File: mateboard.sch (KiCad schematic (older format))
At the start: 2 parts, among them J1 IO1, J2 IO2

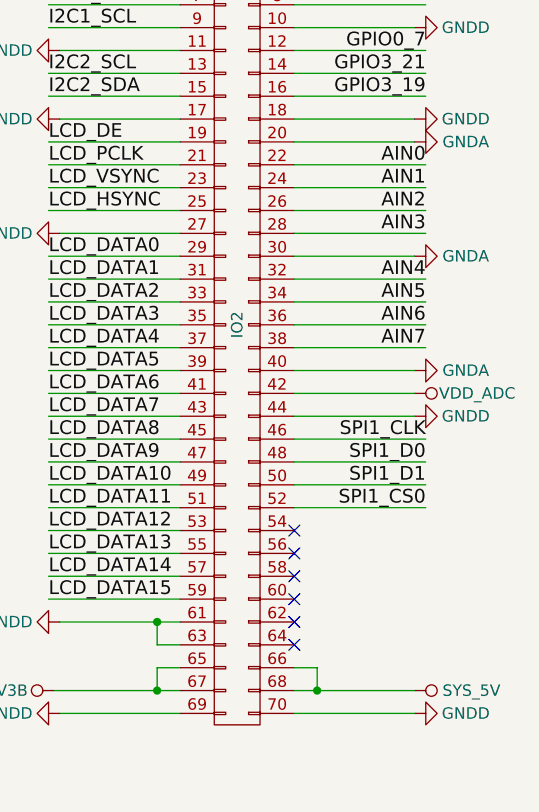
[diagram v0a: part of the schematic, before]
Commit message: erc passed
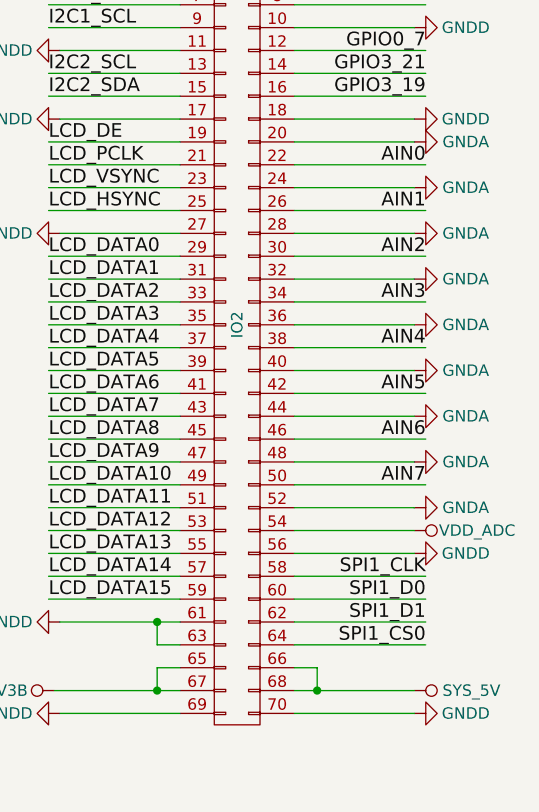
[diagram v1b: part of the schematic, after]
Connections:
- net AIN1: now also J2.26 (P26); no longer J2.24 (P24)
- net AIN2: now also J2.30 (P30); no longer J2.26 (P26)
- net AIN3: now also J2.34 (P34); no longer J2.28 (P28)
- net AIN4: now also J2.38 (P38); no longer J2.32 (P32)
- net AIN5: now also J2.42 (P42); no longer J2.34 (P34)
- net AIN6: now also J2.46 (P46); no longer J2.36 (P36)
- net AIN7: now also J2.50 (P50); no longer J2.38 (P38)
- net GNDA: now also J2.24 (P24), J2.28 (P28), J2.32 (P32), J2.36 (P36), J2.44 (P44), J2.48 (P48), J2.52 (P52); no longer J2.30 (P30)
- net GNDD: now also J2.56 (P56); no longer J2.44 (P44)
- net SPI1_CLK: now also J2.58 (P58); no longer J2.46 (P46)
- net SPI1_CS0: now also J2.64 (P64); no longer J2.52 (P52)
- net SPI1_D0: now also J2.60 (P60); no longer J2.48 (P48)
- net SPI1_D1: now also J2.62 (P62); no longer J2.50 (P50)
- net VDD_ADC: now also J2.54 (P54); no longer J2.42 (P42)
- no-connect marks 6 -> 0
